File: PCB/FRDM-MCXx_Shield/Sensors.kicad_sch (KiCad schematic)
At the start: 3 parts, among them IC1 FXLS8974CF, J1 Conn_01x05_Socket

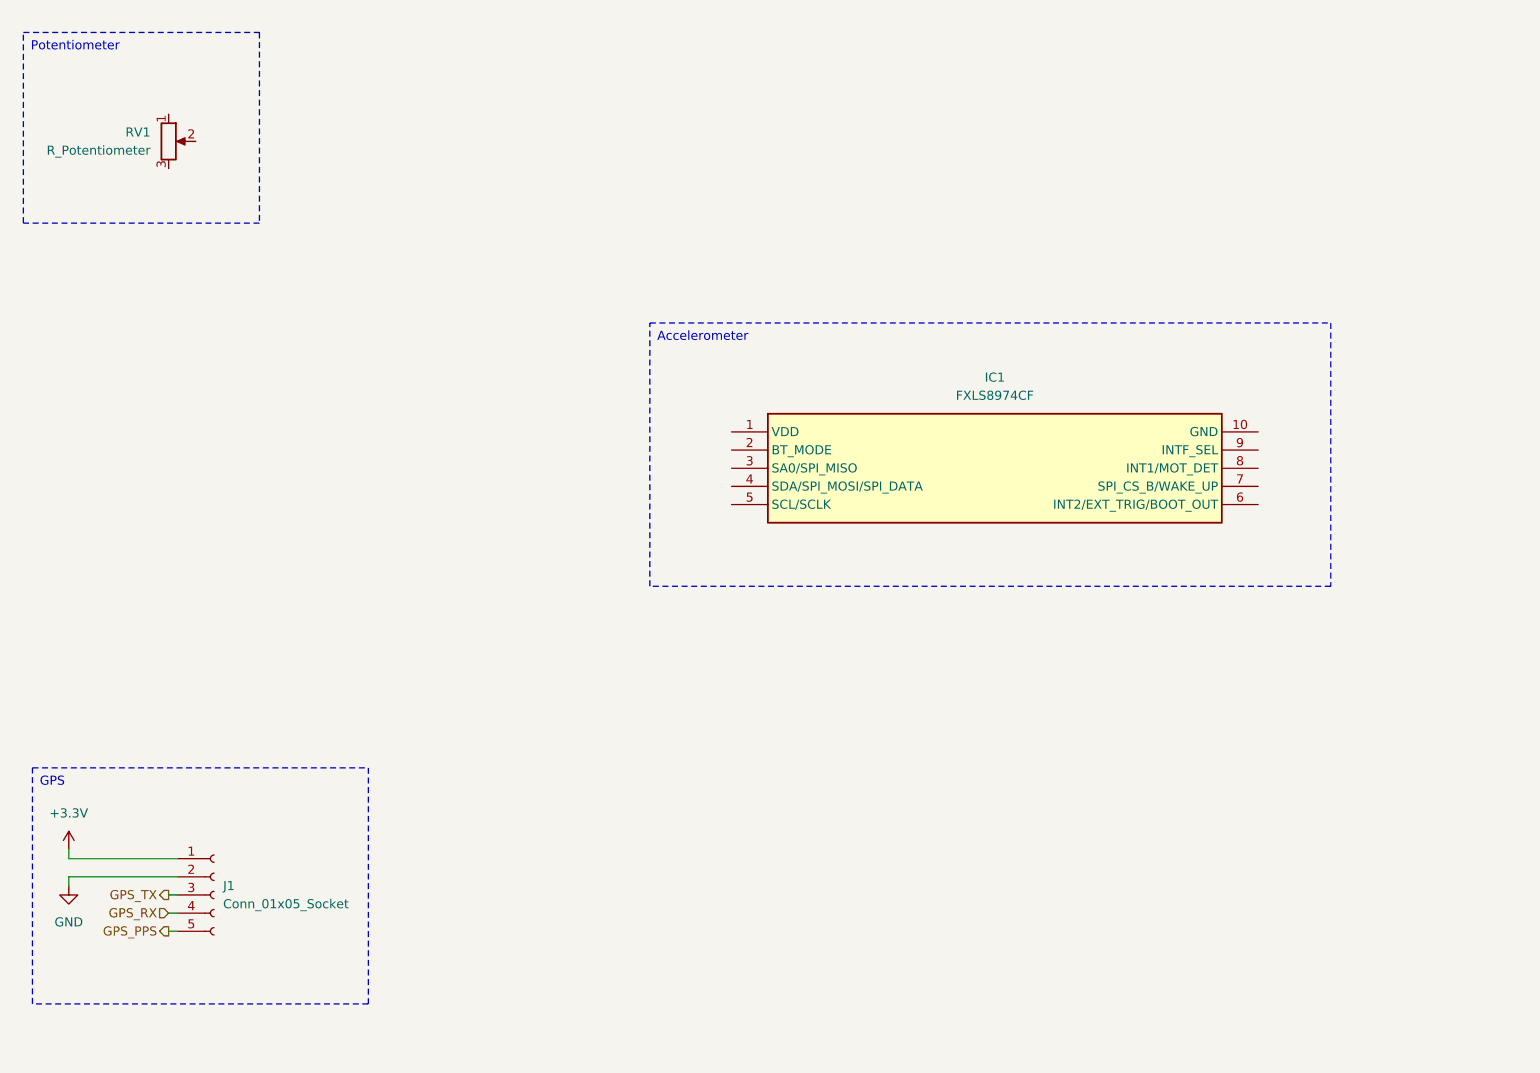
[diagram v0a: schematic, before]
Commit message: Updated schematic
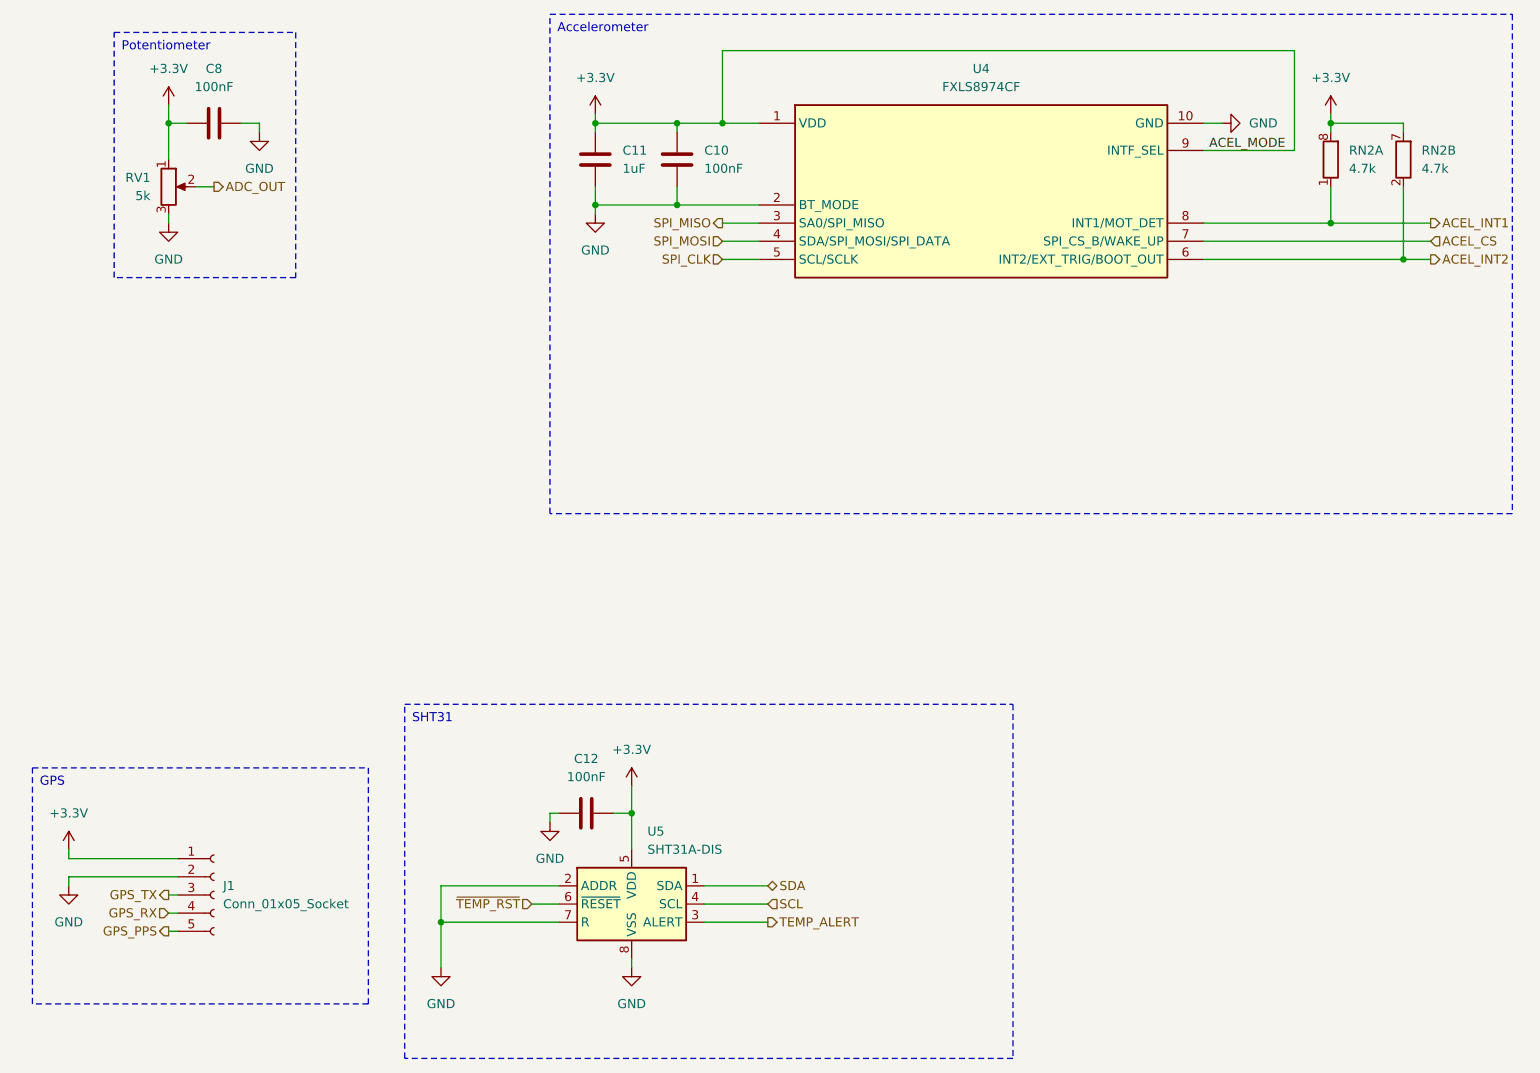
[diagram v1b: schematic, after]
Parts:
- removed IC1: FXLS8974CF, FXLS8974CF, symbol SamacSys_Parts:FXLS8974CF
- added C10, C12, C8: 100nF, Capacitor_SMD:C_0603_1608Metric_Pad1.08x0.95mm_HandSolder, symbol Device:C
- added C11: 1uF, Capacitor_SMD:C_0603_1608Metric_Pad1.08x0.95mm_HandSolder, symbol Device:C
- added RN2: 4.7k, Resistor_SMD:R_Array_Convex_4x0603, symbol Device:R_Pack04_Split
- added U4: FXLS8974CF, FXLS8974CF, symbol SamacSys_Parts:FXLS8974CF
- added U5: SHT31A-DIS, Sensor_Humidity:Sensirion_DFN-8-1EP_2.5x2.5mm_P0.5mm_EP1.1x1.7mm, symbol Sensor_Humidity:SHT31A-DIS
- J1: footprint (none) -> Connector_PinHeader_2.54mm:PinHeader_1x05_P2.54mm_Vertical
- RV1: value R_Potentiometer -> 5k; footprint (none) -> Potentiometer_THT:Potentiometer_Vishay_T73YP_Vertical
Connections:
- net +3.3V: now also RV1.1, C10.1, C11.1, C12.2, C8.1, RN2.7 (R2.2), RN2.8 (R1.2), U4.1 (VDD), U4.9 (INTF_SEL), U5.5 (VDD)
- net GND: now also RV1.3, C10.2, C11.2, C12.1, C8.2, U4.10 (GND), U4.2 (BT_MODE), U5.2 (ADDR), U5.7 (R), U5.8 (VSS), U5.9 (VSS)
- net ADC_OUT: now reaches RV1.2
- new net ACEL_CS: U4.7 (SPI_CS_B/WAKE_UP)
- new net ACEL_INT1: RN2.1 (R1.1), U4.8 (INT1/MOT_DET)
- new net ACEL_INT2: RN2.2 (R2.1), U4.6 (INT2/EXT_TRIG/BOOT_OUT)
- new net SCL: U5.4 (SCL)
- new net SDA: U5.1 (SDA)
- new net SPI_CLK: U4.5 (SCL/SCLK)
- new net SPI_MISO: U4.3 (SA0/SPI_MISO)
- new net SPI_MOSI: U4.4 (SDA/SPI_MOSI/SPI_DATA)
- new net TEMP_ALERT: U5.3 (ALERT)
- new net ~{TEMP_RST}: U5.6 (~{RESET})
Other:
- company: (none) -> HAN
- title: (none) -> Sensors
- moved on the sheet: RV1
